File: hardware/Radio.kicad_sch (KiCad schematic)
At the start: 2 parts, among them U801 RF69, Y801 32_Mhz

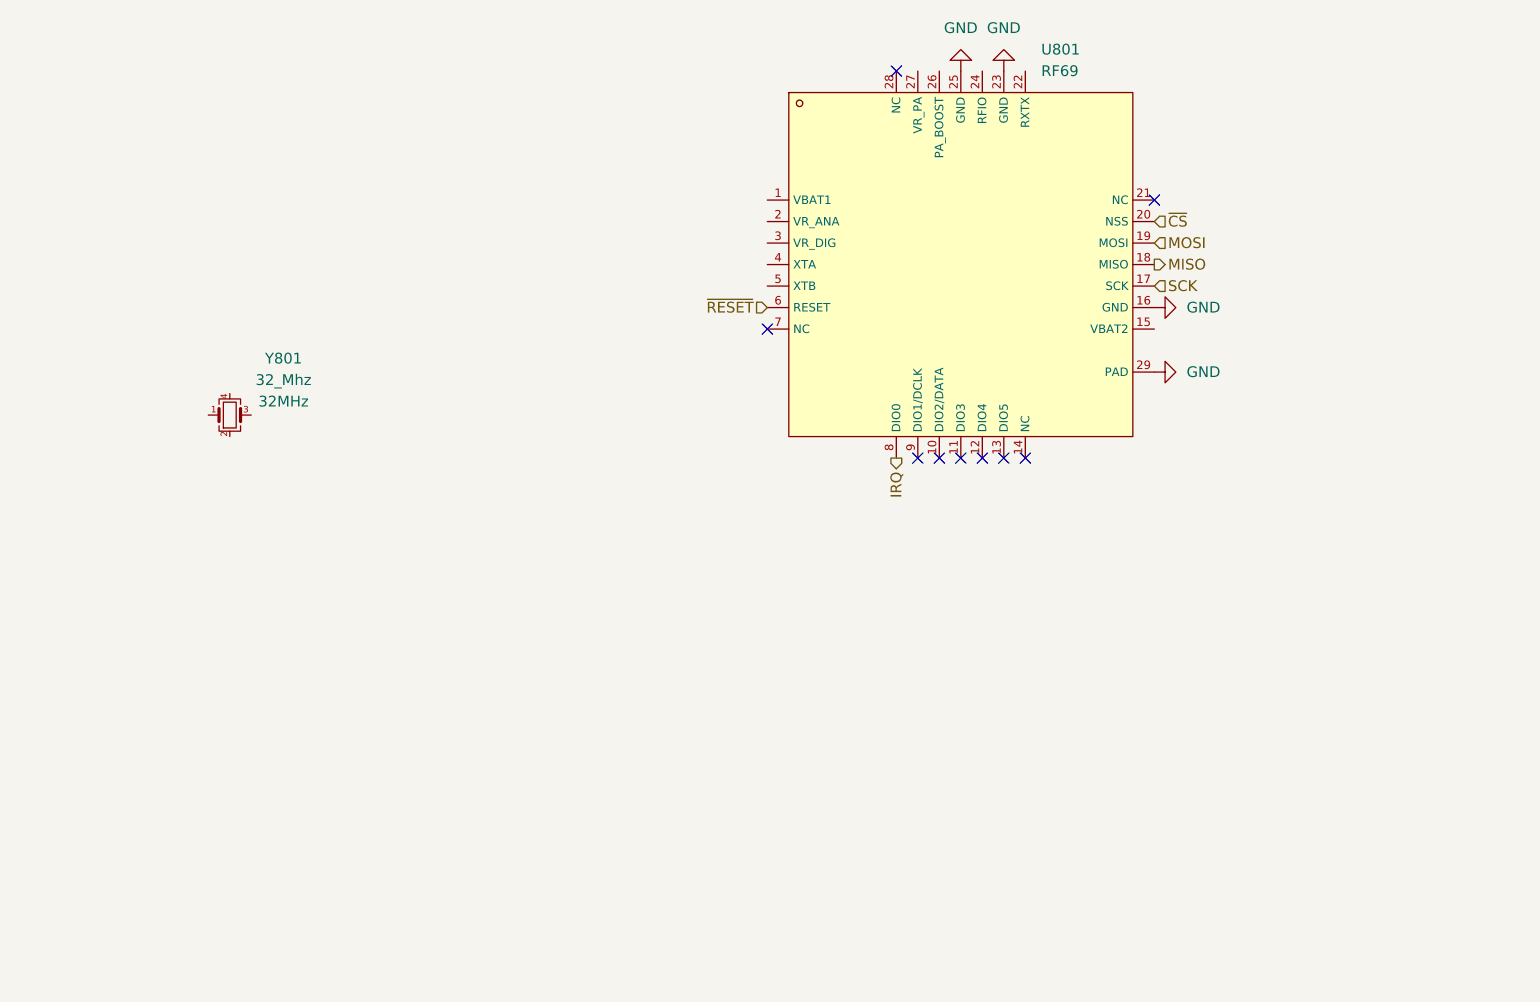
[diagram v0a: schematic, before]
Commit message: Layout updates
Signed-off-by: Connor Rigby <connorr@hey.com>
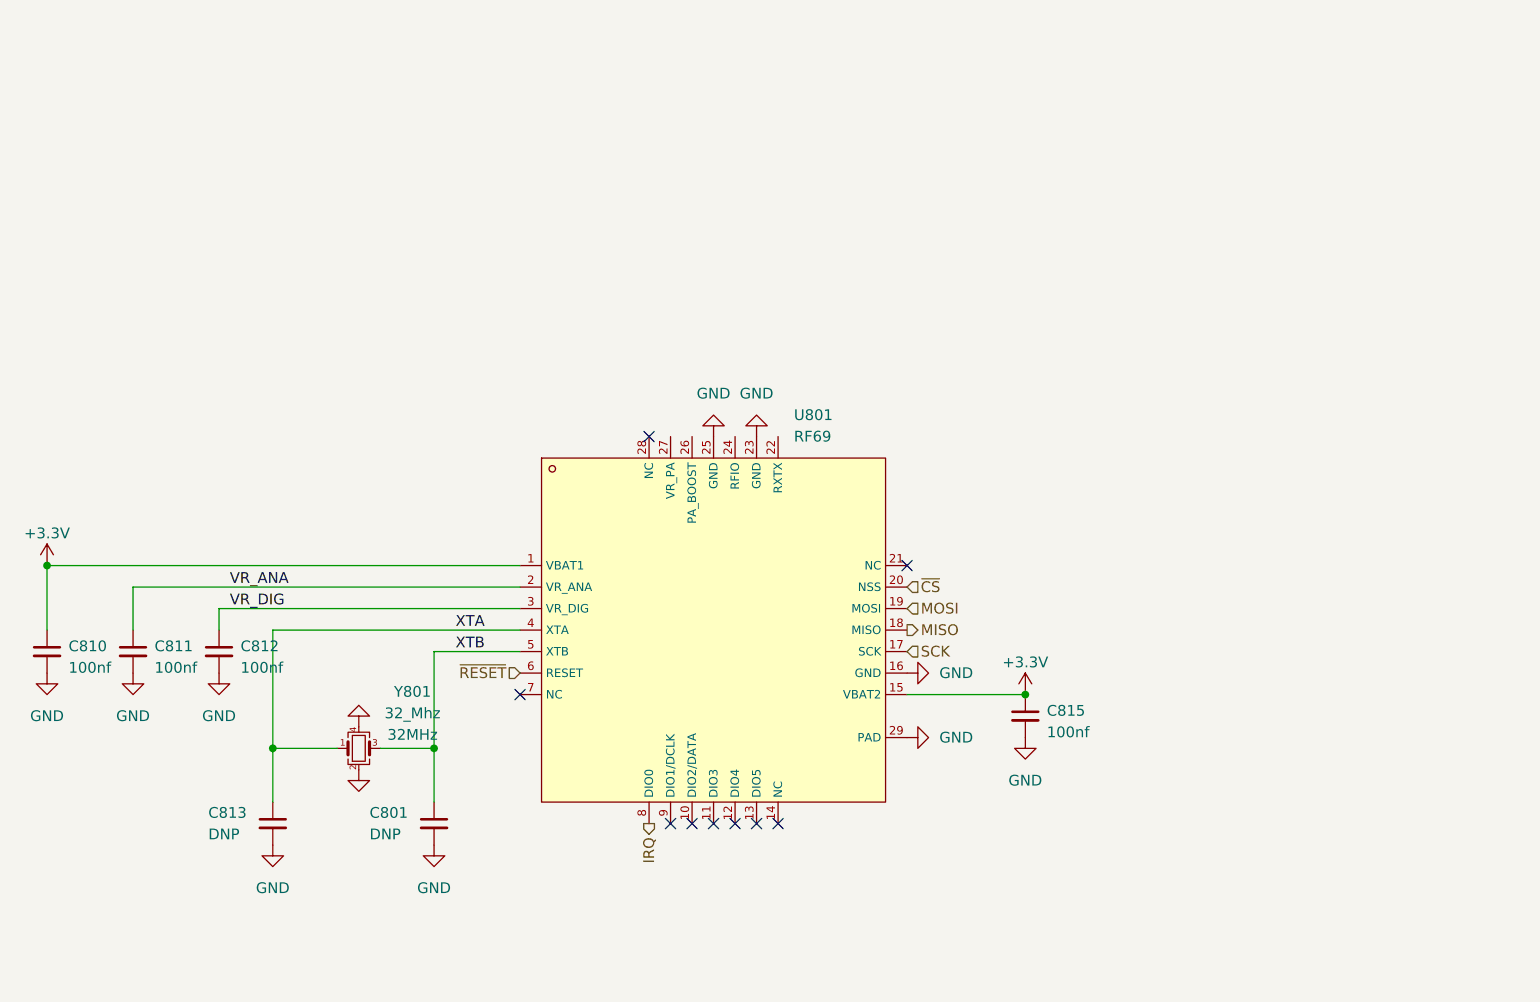
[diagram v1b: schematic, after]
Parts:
- added C801, C813: C_0402_DNP, Capacitor_SMD:C_0402_1005Metric, symbol LCSC_Capacitor:C_0402_DNP
- added C810, C811, C812, C815: C_0402_100nf_X7R, Capacitor_SMD:C_0402_1005Metric, symbol LCSC_Capacitor:C_0402_100nf_X7R
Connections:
- net GND: now also Y801.2, Y801.4, C801.2, C810.2, C811.2, C812.2, C813.2, C815.2
- net XTA: now reaches Y801.1
- net XTA: now also U801.4 (XTA), C813.1
- net XTB: now reaches Y801.3
- net XTB: now also U801.5 (XTB), C801.1
- net +3.3V: now reaches U801.1 (VBAT1)
- net +3.3V: now also U801.15 (VBAT2), C810.1, C815.1
- net VR_ANA: now reaches U801.2 (VR_ANA)
- net VR_ANA: now also C811.1
- net VR_DIG: now reaches U801.3 (VR_DIG)
- net VR_DIG: now also C812.1
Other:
- moved on the sheet: U801, Y801

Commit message: Update layout
Signed-off-by: Connor Rigby <connorr@hey.com>
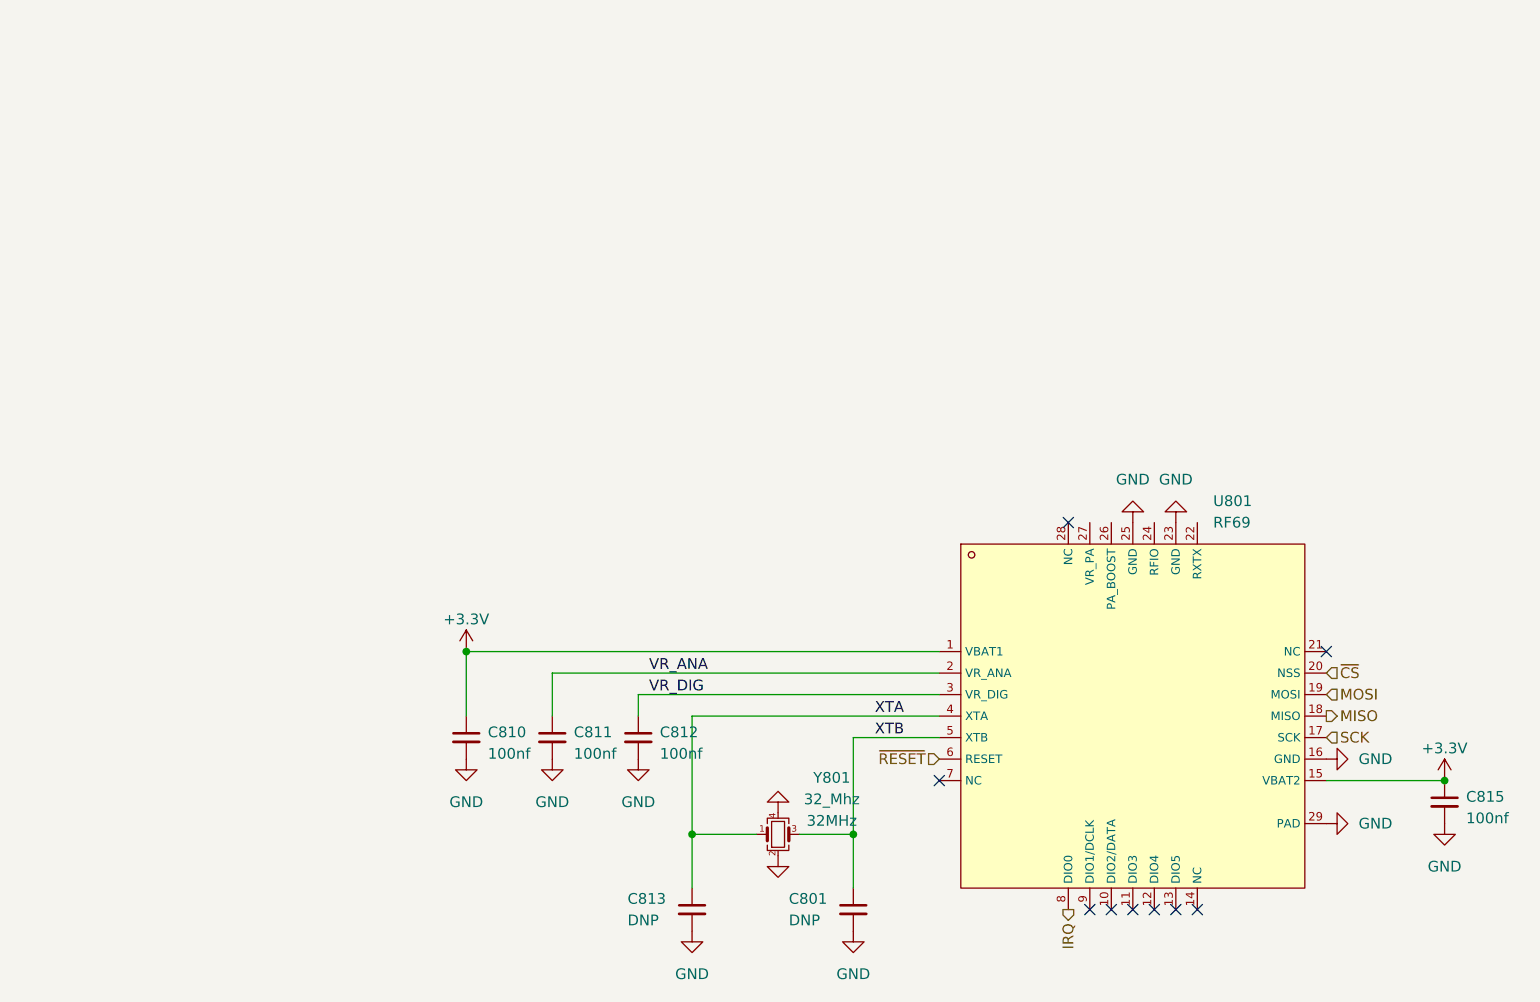
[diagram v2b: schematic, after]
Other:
- moved on the sheet: C801, C810, C811, C812, C813, C815, U801, Y801
